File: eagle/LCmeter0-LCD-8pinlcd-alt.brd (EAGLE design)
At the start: 34 parts, among them IC1 PIC16F876A-X/SP, J1 HD44780-4BIT-8PIN, J2 PIC-UART, J3 PIC-ICSP-ICSP, K2 DS2Y, Q1 20MHz, SW1 SPST, T1 BC547CBE-A, X1 FREQ, X2 L/C

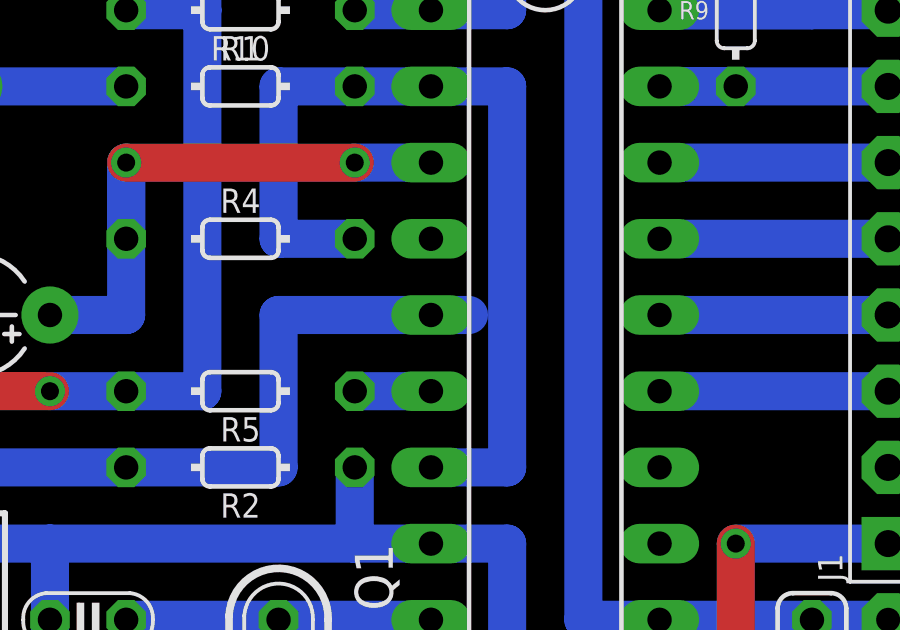
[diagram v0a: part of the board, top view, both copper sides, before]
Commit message: ...
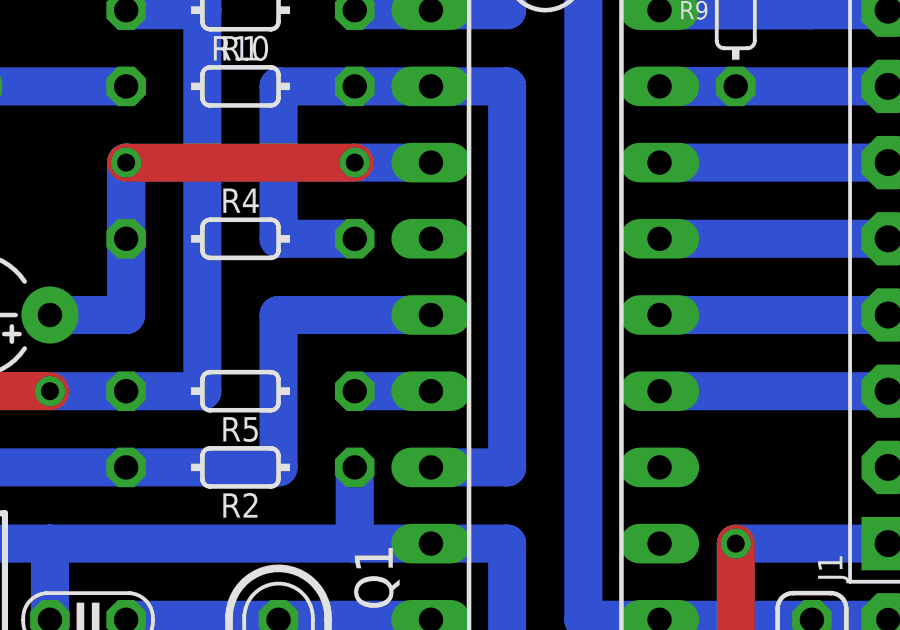
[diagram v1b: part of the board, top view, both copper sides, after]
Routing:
- net A3: track 49.5 -> 48.3 mm
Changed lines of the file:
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@@
 <setting verticaltext="up"/>
 </settings>
-<grid distance="0.1" unitdist="inch" unit="inch" style="dots" multiple="1" display="yes" altdistance="0.05" altunitdist="inch" altunit="inch"/>
+<grid distance="0.05" unitdist="inch" unit="inch" style="dots" multiple="2" display="yes" altdistance="0.005" altunitdist="inch" altunit="inch"/>
 <layers>
 <layer number="1" name="Top" color="4" fill="1" visible="yes" active="yes"/>
+<layer number="16" name="Bottom" color="1" fill="1" visible="yes" active="yes"/>
+<layer number="17" name="Pads" color="2" fill="1" visible="yes" active="yes"/>
+<layer number="18" name="Vias" color="2" fill="1" visible="yes" active="yes"/>
+<layer number="19" name="Unrouted" color="6" fill="1" visible="yes" active="yes"/>
+<layer number="20" name="Dimension" color="24" fill="1" visible="yes" active="yes"/>
+<layer number="21" name="tPlace" color="16" fill="1" visible="yes" active="yes"/>
+<layer number="22" name="bPlace" color="14" fill="1" visible="yes" active="yes"/>
+<layer number="23" name="tOrigins" color="15" fill="1" visible="yes" active="yes"/>
+<layer number="24" name="bOrigins" color="15" fill="1" visible="yes" active="yes"/>
+<layer number="25" name="tNames" color="7" fill="1" visible="no" active="yes"/>
+<layer number="26" name="bNames" color="7" fill="1" visible="no" active="yes"/>
+<layer number="27" name="tValues" color="7" fill="1" visible="no" active="yes"/>
+<layer number="28" name="bValues" color="7" fill="1" visible="no" active="yes"/>
+<layer number="29" name="tStop" color="7" fill="3" visible="no" active="yes"/>
+<layer number="30" name="bStop" color="7" fill="6" visible="no" active="yes"/>
+<layer number="31" name="tCream" color="7" fill="4" visible="no" active="yes"/>
+<layer number="32" name="bCream" color="7" fill="5" visible="no" active="yes"/>
+<layer number="33" name="tFinish" color="6" fill="3" visible="no" active="yes"/>
+<layer number="34" name="bFinish" color="6" fill="6" visible="no" active="yes"/>
+<layer number="35" name="tGlue" color="7" fill="4" visible="no" active="yes"/>
+<layer number="36" name="bGlue" color="7" fill="5" visible="no" active="yes"/>
+<layer number="37" name="tTest" color="7" fill="1" visible="no" active="yes"/>
+<layer number="38" name="bTest" color="7" fill="1" visible="no" active="yes"/>
+<layer number="39" name="tKeepout" color="4" fill="11" visible="no" active="yes"/>
+<layer number="40" name="bKeepout" color="1" fill="11" visible="no" active="yes"/>
+<layer number="41" name="tRestrict" color="4" fill="10" visible="no" active="yes"/>
+<layer number="42" name="bRestrict" color="1" fill="10" visible="no" active="yes"/>
+<layer number="43" name="vRestrict" color="2" fill="10" visible="no" active="yes"/>
+<layer number="44" name="Drills" color="7" fill="1" visible="no" active="yes"/>
+<layer number="45" name="Holes" color="7" fill="1" visible="yes" active="yes"/>
+<layer number="46" name="Milling" color="3" fill="1" visible="no" active="yes"/>
+<layer number="47" name="Measures" color="7" fill="1" visible="no" active="yes"/>
+<layer number="48" name="Document" color="7" fill="1" visible="no" active="yes"/>
+<layer number="49" name="Reference" color="7" fill="1" visible="no" active="yes"/>
+<layer number="51" name="tDocu" color="6" fill="1" visible="yes" active="yes"/>
+<layer number="52" name="bDocu" color="7" fill="1" visible="no" active="yes"/>
+<layer number="91" name="Nets" color="2" fill="1" visible="no" active="no"/>
+<layer number="92" name="Busses" color="1" fill="1" visible="no" active="no"/>
+<layer number="93" name="Pins" color="2" fill="1" visible="no" active="no"/>
+<layer number="94" name="Symbols" color="4" fill="1" visible="no" active="no"/>
+<layer number="95" name="Names" color="7" fill="1" visible="no" active="no"/>
+<layer number="96" name="Values" color="7" fill="1" visible="no" active="no"/>
 <layer number="2" name="Route2" color="1" fill="3" visible="no" active="no"/>
 <layer number="3" name="Route3" color="4" fill="3" visible="no" active="no"/>
@@
 <layer number="14" name="Route14" color="1" fill="6" visible="no" active="no"/>
 <layer number="15" name="Route15" color="4" fill="6" visible="no" active="no"/>
-<layer number="16" name="Bottom" color="1" fill="1" visible="yes" active="yes"/>
-<layer number="17" name="Pads" color="2" fill="1" visible="yes" active="yes"/>
-<layer number="18" name="Vias" color="2" fill="1" visible="yes" active="yes"/>
-<layer number="19" name="Unrouted" color="6" fill="1" visible="yes" active="yes"/>
-<layer number="20" name="Dimension" color="15" fill="1" visible="yes" active="yes"/>
-<layer number="21" name="tPlace" color="7" fill="1" visible="yes" active="yes"/>
-<layer number="22" name="bPlace" color="7" fill="1" visible="yes" active="yes"/>
-<layer number="23" name="tOrigins" color="15" fill="1" visible="yes" active="yes"/>
-<layer number="24" name="bOrigins" color="15" fill="1" visible="yes" active="yes"/>
-<layer number="25" name="tNames" color="7" fill="1" visible="yes" active="yes"/>
-<layer number="26" name="bNames" color="7" fill="1" visible="yes" active="yes"/>
-<layer number="27" name="tValues" color="7" fill="1" visible="yes" active="yes"/>
-<layer number="28" name="bValues" color="7" fill="1" visible="yes" active="yes"/>
-<layer number="29" name="tStop" color="7" fill="3" visible="no" active="yes"/>
-<layer number="30" name="bStop" color="7" fill="6" visible="no" active="yes"/>
-<layer number="31" name="tCream" color="7" fill="4" visible="no" active="yes"/>
-<layer number="32" name="bCream" color="7" fill="5" visible="no" active="yes"/>
-<layer number="33" name="tFinish" color="6" fill="3" visible="no" active="yes"/>
-<layer number="34" name="bFinish" color="6" fill="6" visible="no" active="yes"/>
-<layer number="35" name="tGlue" color="7" fill="4" visible="no" active="yes"/>
-<layer number="36" name="bGlue" color="7" fill="5" visible="no" active="yes"/>
-<layer number="37" name="tTest" color="7" fill="1" visible="no" active="yes"/>
-<layer number="38" name="bTest" color="7" fill="1" visible="no" active="yes"/>
-<layer number="39" name="tKeepout" color="4" fill="11" visible="no" active="yes"/>
-<layer number="40" name="bKeepout" color="1" fill="11" visible="no" active="yes"/>
-<layer number="41" name="tRestrict" color="4" fill="10" visible="no" active="yes"/>
-<layer number="42" name="bRestrict" color="1" fill="10" visible="no" active="yes"/>
-<layer number="43" name="vRestrict" color="2" fill="10" visible="yes" active="yes"/>
-<layer number="44" name="Drills" color="7" fill="1" visible="no" active="yes"/>
-<layer number="45" name="Holes" color="7" fill="1" visible="no" active="yes"/>
-<layer number="46" name="Milling" color="3" fill="1" visible="no" active="yes"/>
-<layer number="47" name="Measures" color="7" fill="1" visible="no" active="yes"/>
-<layer number="48" name="Document" color="7" fill="1" visible="no" active="yes"/>
-<layer number="49" name="Reference" color="7" fill="1" visible="no" active="yes"/>
-<layer number="51" name="tDocu" color="7" fill="1" visible="yes" active="yes"/>
-<layer number="52" name="bDocu" color="7" fill="1" visible="yes" active="yes"/>
 <layer number="90" name="Modules" color="5" fill="10" visible="no" active="no"/>
-<layer number="91" name="Nets" color="2" fill="1" visible="no" active="no"/>
-<layer number="92" name="Busses" color="1" fill="1" visible="no" active="no"/>
-<layer number="93" name="Pins" color="2" fill="1" visible="no" active="no"/>
-<layer number="94" name="Symbols" color="4" fill="1" visible="no" active="no"/>
-<layer number="95" name="Names" color="7" fill="1" visible="no" active="no"/>
-<layer number="96" name="Values" color="7" fill="1" visible="no" active="no"/>
 <layer number="97" name="Info" color="7" fill="1" visible="no" active="no"/>
 <layer number="98" name="Guide" color="6" fill="1" visible="no" active="no"/>
 <layer number="99" name="SpiceOrder" color="5" fill="1" visible="no" active="no"/>
-<layer number="250" name="trash" color="7" fill="1" visible="yes" active="yes"/>
+<layer number="250" name="trash" color="7" fill="1" visible="no" active="no"/>
 </layers>
 <board>
@@
 <wire x1="33.02" y1="25.4" x2="33.02" y2="30.48" width="1.27" layer="16"/>
 <wire x1="33.02" y1="30.48" x2="38.1" y2="30.48" width="1.27" layer="16"/>
-<wire x1="39.37" y1="30.48" x2="38.1" y2="30.48" width="1.27" layer="16"/>
 <wire x1="27.94" y1="38.1" x2="22.86" y2="38.1" width="1.27" layer="16"/>
 <wire x1="22.86" y1="38.1" x2="22.86" y2="43.18" width="1.27" layer="16"/>
